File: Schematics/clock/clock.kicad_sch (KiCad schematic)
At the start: 55 parts, among them J2 Power, SW1 Step, SW2 Mode, SW3 Reset, U1 74LS04, U10 ATmega328-P, U12 5641AS, U2 LM555, U3 74LS32, U4 74LS08, U5 LM555, U6 LM555, U7 LM555, U8 74LS08, U9 74HC14

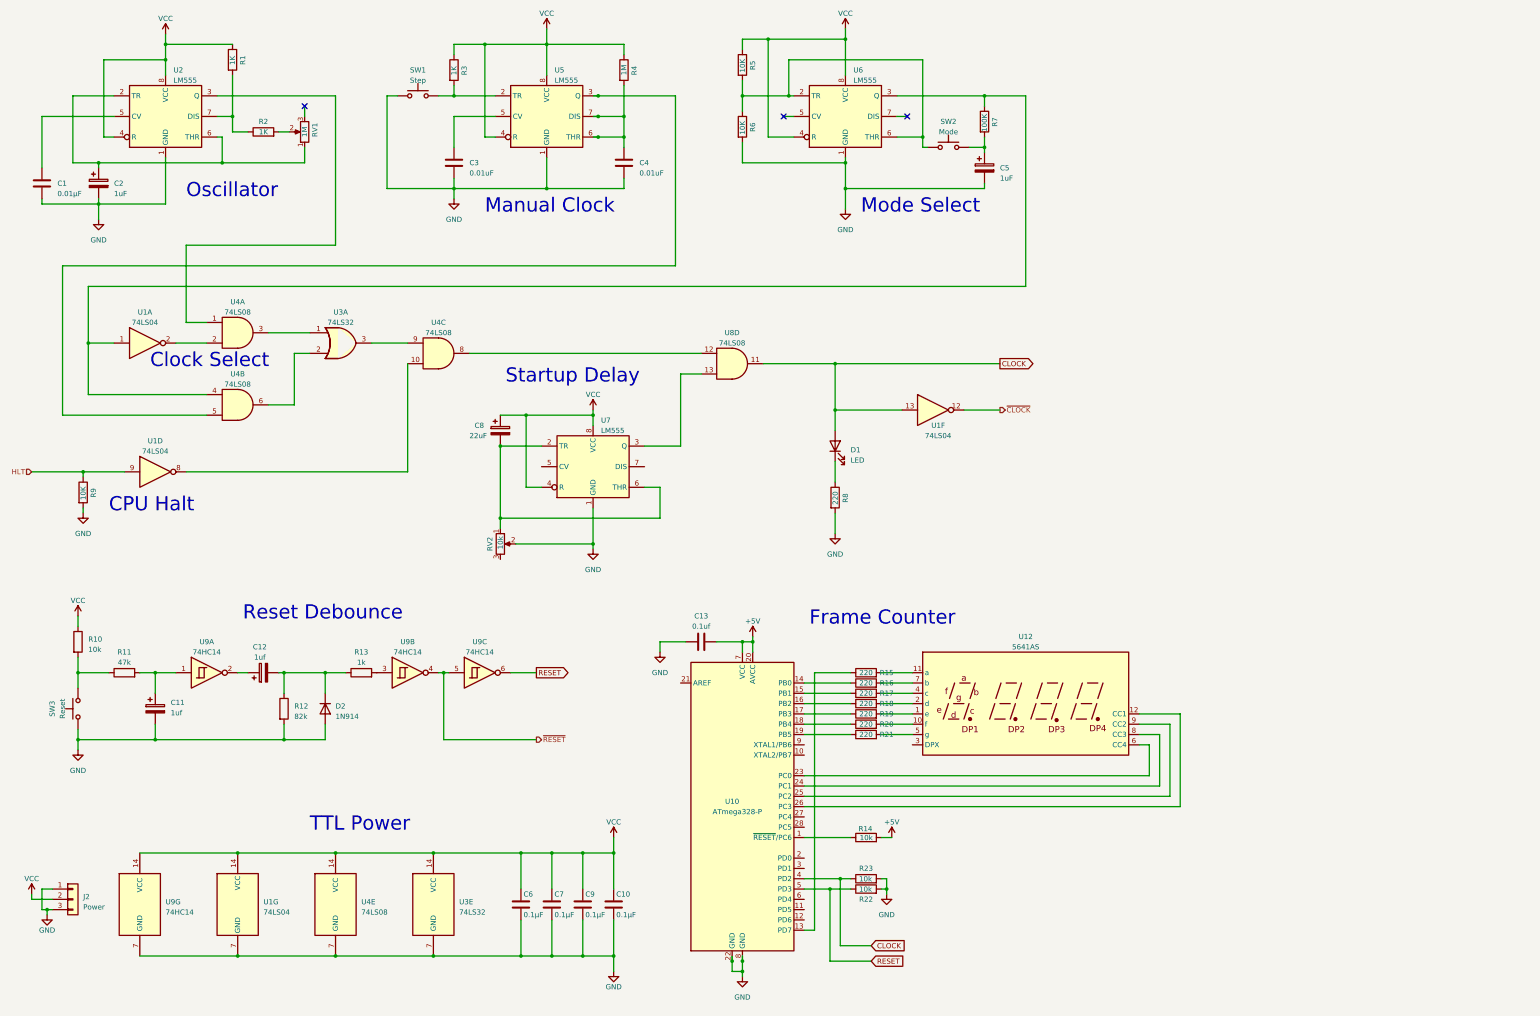
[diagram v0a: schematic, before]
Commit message: Updates
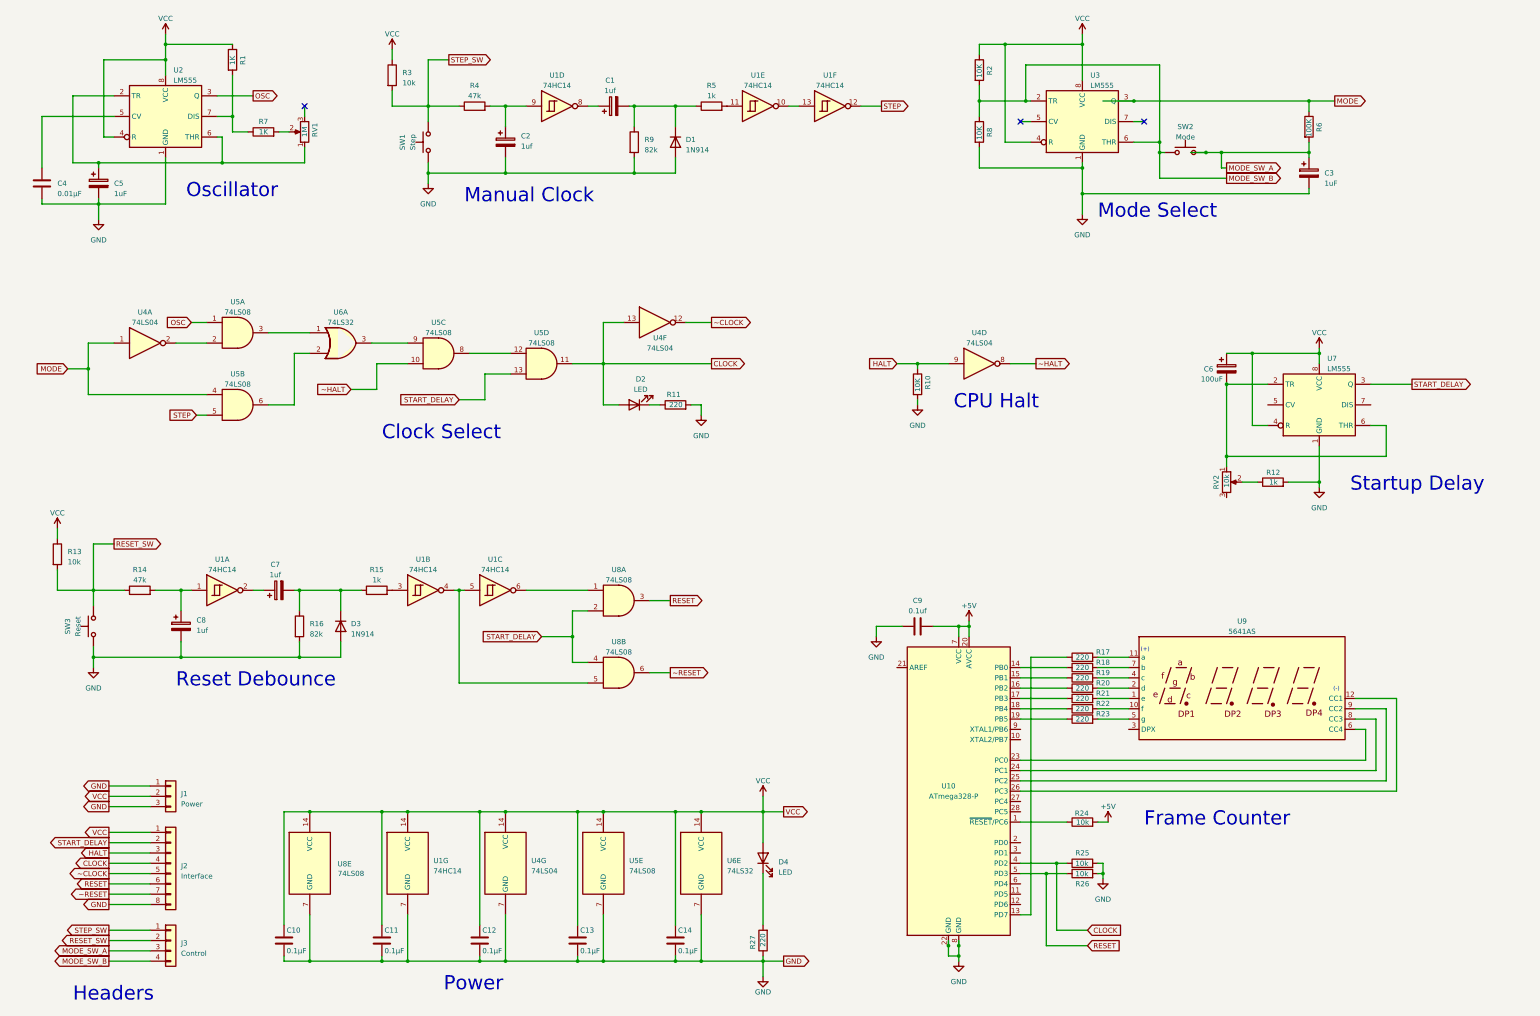
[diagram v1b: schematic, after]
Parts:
- removed C3, C4: 0.01uF, symbol Device:C
- removed C8: 22uF, symbol Device:C_Polarized
- removed U5: LM555, Package_SO:SOIC-8_3.9x4.9mm_P1.27mm, symbol Timer:LM555xM
- added C1, C2: 1uf, symbol Device:C_Polarized
- added C10: 0.1µF, Capacitor_THT:C_Disc_D4.3mm_W1.9mm_P5.00mm, symbol Device:C
- added C6: 100uF, symbol Device:C_Polarized
- added D1: 1N914, Diode_THT:D_DO-35_SOD27_P7.62mm_Horizontal, symbol Diode:1N914
- added D4: LED, symbol Device:LED
- added J2: Interface, symbol Connector_Generic:Conn_01x08
- added J3: Control, symbol Connector_Generic:Conn_01x04
- added R12, R5: 1k, symbol Device:R
- added R27: 220, symbol Device:R
- added R9: 82k, symbol Device:R
- added unit 6 of U1
- added unit 4 of U1
- added unit 5 of U1
- added U8: 74LS08, symbol 74xx:74LS08
- R3: value 1K -> 10k
- R4: value 1M -> 47k
- renumbered C6 to C11, C7 to C12, C9 to C13, C10 to C14, C5 to C3, C1 to C4, C2 to C5, C12 to C7, C11 to C8, C13 to C9, D1 to D2, D2 to D3, J2 to J1, R9 to R10, R8 to R11, R10 to R13, R11 to R14, R13 to R15, R12 to R16, R15 to R17, R16 to R18, R17 to R19, R5 to R2, R18 to R20, R19 to R21, R20 to R22, R21 to R23, R14 to R24, R23 to R25, R22 to R26, R7 to R6, R2 to R7, R6 to R8, U9 to U1, U6 to U3, U1 to U4, U4 to U5, U8 to U5, U3 to U6, U12 to U9
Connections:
- net CLOCK: now also J2.4 (Pin_4)
- net GND: now also C10.2, C2.2, D1.2 (A), J2.8 (Pin_8), R12.2, R27.1, R9.2, U8.7 (GND); no longer RV2.2
- net RESET: now also J2.6 (Pin_6), U8.3; no longer U1.6
- net VCC: now also C10.1, C6.1, D4.2 (A), J2.1 (Pin_1), U8.14 (VCC); no longer R4.1
- net ~HALT: now reaches U4.8, U5.10
- net MODE_SW_B: now reaches R2.2, R8.1, SW2.1, U3.2 (TR), U3.6 (THR)
- net MODE_SW_B: now also J3.4 (Pin_4)
- net at RV2.1, U7.2 (TR), U7.6 (THR): now also C6.2
- net STEP_SW: now reaches R3.2, SW1.2
- net STEP_SW: now also R4.1, J3.1 (Pin_1)
- net STEP: now reaches U5.5
- net STEP: now also U1.12
- net at R4.2: now also C2.1, U1.9
- net MODE_SW_A: now reaches C3.1, R6.2, SW2.2
- net MODE_SW_A: now also J3.3 (Pin_3)
- net MODE: now reaches R6.1, U3.3 (Q), U4.1, U5.4
- net START_DELAY: now reaches U5.13, U7.3 (Q)
- net START_DELAY: now also J2.2 (Pin_2), U8.2, U8.4
- net RESET_SW: now reaches R13.2, R14.1, SW3.2
- net RESET_SW: now also J3.2 (Pin_2)
- net OSC: now reaches U2.3 (Q), U5.1
- net HLT renamed HALT
- net HALT: now also J2.3 (Pin_3)
- net ~{CLOCK} renamed ~CLOCK
- net ~CLOCK: now also J2.5 (Pin_5)
- net ~{RESET}: no longer names the net of U1.4, U1.5
- net ~{RESET}: now also U8.5
- new net: R12.1, RV2.2
- new net: D4.1 (K), R27.2
- new net: U1.10, U1.13
- new net: C1.2, D1.1 (K), R5.1, R9.1
- new net: U1.6, U8.1
- new net: C1.1, U1.8
- new net: R5.2, U1.11
- new net ~RESET: J2.7 (Pin_7), U8.6
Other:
- note added: "(+)"
- note added: "(-)"
- note added: "Headers"
- note added: "Power"
- note removed: "TTL Power"
- moved on the sheet: C11, C12, C13, C14, C3, C7, C8, C9, D2, D3, J1, R10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
